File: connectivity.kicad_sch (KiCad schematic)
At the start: 52 parts, among them CN1 GPS_Port, CN2 SM06B-GHS-TB(LF)(SN), Con2 DS1023-1X2SF11, Con3 DS1023-1X10SF11, Con4 DS1023-1X6SF11, J1 USB_C_Receptacle, J10 DS1023-1X5SF11, J11 DS1023-1X5SF11, J12 DS1023-1X5SF11, J13 DS1023-1X5SF11, J14 DS1023-1X5SF11, J2 DS1023-1X9S21, J3 DS1023-1X7SF11, J4 DS1023-1X8SF11, J5 DS1023-1X6SF11, J6 DS1023-1X6SF11, J7 DS1023-1X8SF11, J8 DS1023-1X8SF11, J9 DS1023-1X5SF11, U3 FT232RL, con1 DS1023-1X3SF11

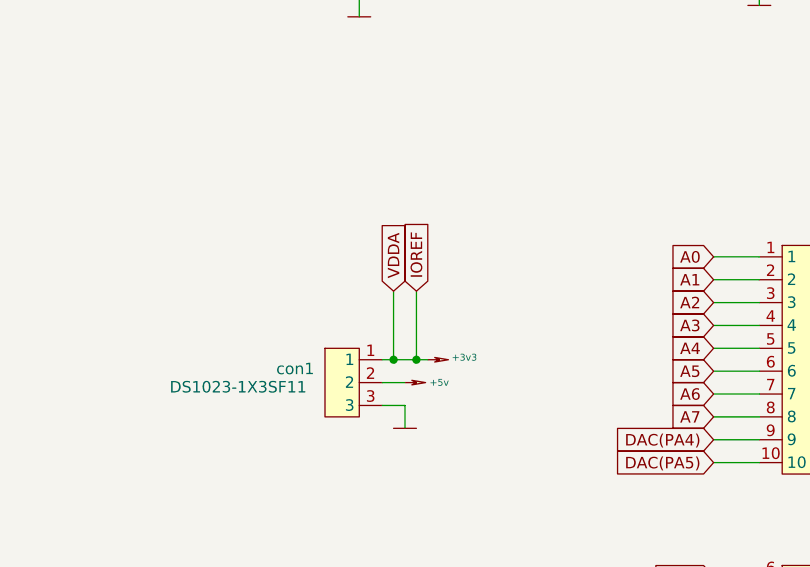
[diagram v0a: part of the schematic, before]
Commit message: Add files via upload
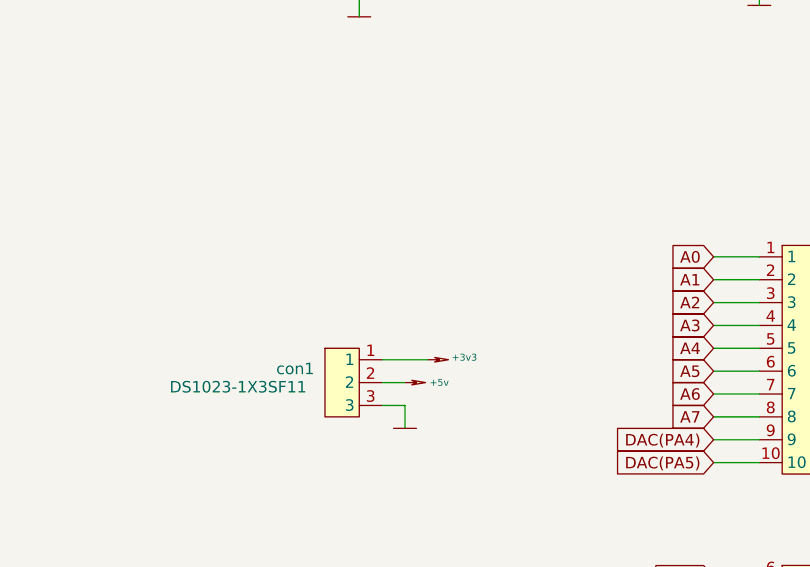
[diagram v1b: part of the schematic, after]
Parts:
- C40: footprint (none) -> Capacitor_SMD:C_0603_1608Metric
- Con2: footprint Connector_PinHeader_1.00mm:PinHeader_1x02_P1.00mm_Vertical -> Connector_PinHeader_2.54mm:PinHeader_1x02_P2.54mm_Vertical
- Con3: footprint Connector_PinHeader_1.00mm:PinHeader_1x10_P1.00mm_Vertical -> Connector_PinHeader_2.54mm:PinHeader_1x10_P2.54mm_Vertical
- Con4, J5, J6: footprint Connector_PinHeader_1.00mm:PinHeader_1x06_P1.00mm_Vertical -> Connector_PinHeader_2.54mm:PinHeader_1x06_P2.54mm_Vertical
- DynamixelCon1, con1: footprint Connector_PinHeader_1.00mm:PinHeader_1x03_P1.00mm_Vertical -> Connector_PinHeader_2.54mm:PinHeader_1x03_P2.54mm_Vertical
- J2: footprint Connector_PinHeader_1.00mm:PinHeader_1x09_P1.00mm_Vertical -> Connector_PinHeader_2.54mm:PinHeader_1x09_P2.54mm_Vertical
- J3: footprint Connector_PinHeader_1.00mm:PinHeader_1x07_P1.00mm_Vertical -> Connector_PinHeader_2.54mm:PinHeader_1x07_P2.54mm_Vertical
- J4, J7, J8: footprint Connector_PinHeader_1.00mm:PinHeader_1x08_P1.00mm_Vertical -> Connector_PinHeader_2.54mm:PinHeader_1x08_P2.54mm_Vertical
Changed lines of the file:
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@@
 	)
 	(junction
-		(at 275.59 100.33)
-		(diameter 0)
-		(color 0 0 0 0)
-	)
-	(junction
 		(at 130.81 204.47)
 		(diameter 0)
@@
 	)
 	(junction
-		(at 273.05 100.33)
-		(diameter 0)
-		(color 0 0 0 0)
-	)
-	(junction
 		(at 53.34 66.04)
 		(diameter 0)
@@
 	(wire
 		(pts
-			(xy 271.78 100.33) (xy 273.05 100.33)
-		)
-		(stroke
-			(width 0)
-			(type default)
-		)
-	)
-	(wire
-		(pts
 			(xy 209.55 58.42) (xy 200.66 58.42)
 		)
@@
 	(wire
 		(pts
-			(xy 275.59 92.71) (xy 275.59 100.33)
-		)
-		(stroke
-			(width 0)
-			(type default)
-		)
-	)
-	(wire
-		(pts
 			(xy 218.44 53.34) (xy 217.17 53.34)
 		)
@@
 	(wire
 		(pts
-			(xy 273.05 92.71) (xy 273.05 100.33)
-		)
-		(stroke
-			(width 0)
-			(type default)
-		)
-	)
-	(wire
-		(pts
 			(xy 209.55 52.07) (xy 209.55 58.42)
 		)
@@
 	(wire
 		(pts
-			(xy 275.59 100.33) (xy 276.86 100.33)
+			(xy 271.78 100.33) (xy 276.86 100.33)
 		)
 		(stroke
@@
 	(wire
 		(pts
-			(xy 273.05 100.33) (xy 275.59 100.33)
-		)
-		(stroke
-			(width 0)
-			(type default)
-		)
-	)
-	(wire
-		(pts
 			(xy 313.69 137.16) (xy 308.61 137.16)
 		)
@@
 		)
 	)
-	(global_label "VDDA"
-		(shape input)
-		(at 273.05 92.71 90)
-		(fields_autoplaced yes)
-		(effects
-			(font
-				(size 1.27 1.27)
-			)
-			(justify left)
-		)
-		(property "Intersheetrefs" "${INTERSHEET_REFS}"
-			(at 273.05 85.0076 90)
-			(hide yes)
-			(show_name no)
-			(do_not_autoplace no)
-			(effects
-				(font
-					(size 1.27 1.27)
-				)
-				(justify left)
-			)
-		)
-	)
 	(global_label "UART8_TX"
 		(shape input)
@@
 		)
 	)
-	(global_label "IOREF"
-		(shape input)
-		(at 275.59 92.71 90)
-		(effects
-			(font
-				(size 1.27 1.27)
-			)
-			(justify left)
-		)
-		(property "Intersheetrefs" "${INTERSHEET_REFS}"
-			(at 275.59 92.71 90)
-			(hide yes)
-			(show_name no)
-			(do_not_autoplace no)
-			(effects
-				(font
-					(size 1.27 1.27)
-				)
-			)
-		)
-	)
 	(global_label "SWDIO"
 		(shape input)
@@
 			)
 		)
-		(property "Footprint" "Connector_PinHeader_1.00mm:PinHeader_1x06_P1.00mm_Vertical"
+		(property "Footprint" "Connector_PinHeader_2.54mm:PinHeader_1x06_P2.54mm_Vertical"
 			(at 255.27 219.71 0)
 			(hide yes)
@@
 			)
 		)
-		(property "Footprint" ""
+		(property "Footprint" "Capacitor_SMD:C_0603_1608Metric"
 			(at 313.69 52.07 0)
 			(hide yes)
@@
 			)
 		)
-		(property "Footprint" "Connector_PinHeader_1.00mm:PinHeader_1x03_P1.00mm_Vertical"
+		(property "Footprint" "Connector_PinHeader_2.54mm:PinHeader_1x03_P2.54mm_Vertical"
 			(at 267.97 102.87 0)
 			(hide yes)
@@
 			)
 		)
-		(property "Footprint" "Connector_PinHeader_1.00mm:PinHeader_1x02_P1.00mm_Vertical"
+		(property "Footprint" "Connector_PinHeader_2.54mm:PinHeader_1x02_P2.54mm_Vertical"
 			(at 316.23 153.67 0)
 			(hide yes)
@@
 			)
 		)
-		(property "Footprint" "Connector_PinHeader_1.00mm:PinHeader_1x06_P1.00mm_Vertical"
+		(property "Footprint" "Connector_PinHeader_2.54mm:PinHeader_1x06_P2.54mm_Vertical"
 			(at 317.5 124.46 0)
 			(hide yes)
@@
 			)
 		)
-		(property "Footprint" "Connector_PinHeader_1.00mm:PinHeader_1x07_P1.00mm_Vertical"
+		(property "Footprint" "Connector_PinHeader_2.54mm:PinHeader_1x07_P2.54mm_Vertical"
 			(at 255.27 152.4 0)
 			(hide yes)
@@
 			)
 		)
-		(property "Footprint" "Connector_PinHeader_1.00mm:PinHeader_1x08_P1.00mm_Vertical"
+		(property "Footprint" "Connector_PinHeader_2.54mm:PinHeader_1x08_P2.54mm_Vertical"
 			(at 255.27 171.45 0)
 			(hide yes)
@@
 			)
 		)
-		(property "Footprint" "Connector_PinHeader_1.00mm:PinHeader_1x09_P1.00mm_Vertical"
+		(property "Footprint" "Connector_PinHeader_2.54mm:PinHeader_1x09_P2.54mm_Vertical"
 			(at 214.63 181.61 0)
 			(hide yes)
@@
 			)
 		)
-		(property "Footprint" "Connector_PinHeader_1.00mm:PinHeader_1x06_P1.00mm_Vertical"
+		(property "Footprint" "Connector_PinHeader_2.54mm:PinHeader_1x06_P2.54mm_Vertical"
 			(at 255.27 203.2 0)
 			(hide yes)
@@
 			)
 		)
-		(property "Footprint" "Connector_PinHeader_1.00mm:PinHeader_1x03_P1.00mm_Vertical"
+		(property "Footprint" "Connector_PinHeader_2.54mm:PinHeader_1x03_P2.54mm_Vertical"
 			(at 340.36 43.18 0)
 			(hide yes)
@@
 			)
 		)
-		(property "Footprint" "Connector_PinHeader_1.00mm:PinHeader_1x08_P1.00mm_Vertical"
+		(property "Footprint" "Connector_PinHeader_2.54mm:PinHeader_1x08_P2.54mm_Vertical"
 			(at 304.8 196.85 0)
 			(hide yes)
@@
 			)
 		)
-		(property "Footprint" "Connector_PinHeader_1.00mm:PinHeader_1x08_P1.00mm_Vertical"
+		(property "Footprint" "Connector_PinHeader_2.54mm:PinHeader_1x08_P2.54mm_Vertical"
 			(at 304.8 173.99 0)
 			(hide yes)
@@
 			)
 		)
-		(property "Footprint" "Connector_PinHeader_1.00mm:PinHeader_1x10_P1.00mm_Vertical"
+		(property "Footprint" "Connector_PinHeader_2.54mm:PinHeader_1x10_P2.54mm_Vertical"
 			(at 317.5 100.33 0)
 			(hide yes)
